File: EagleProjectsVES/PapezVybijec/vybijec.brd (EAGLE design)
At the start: 55.9 x 40.9 mm, 32 parts

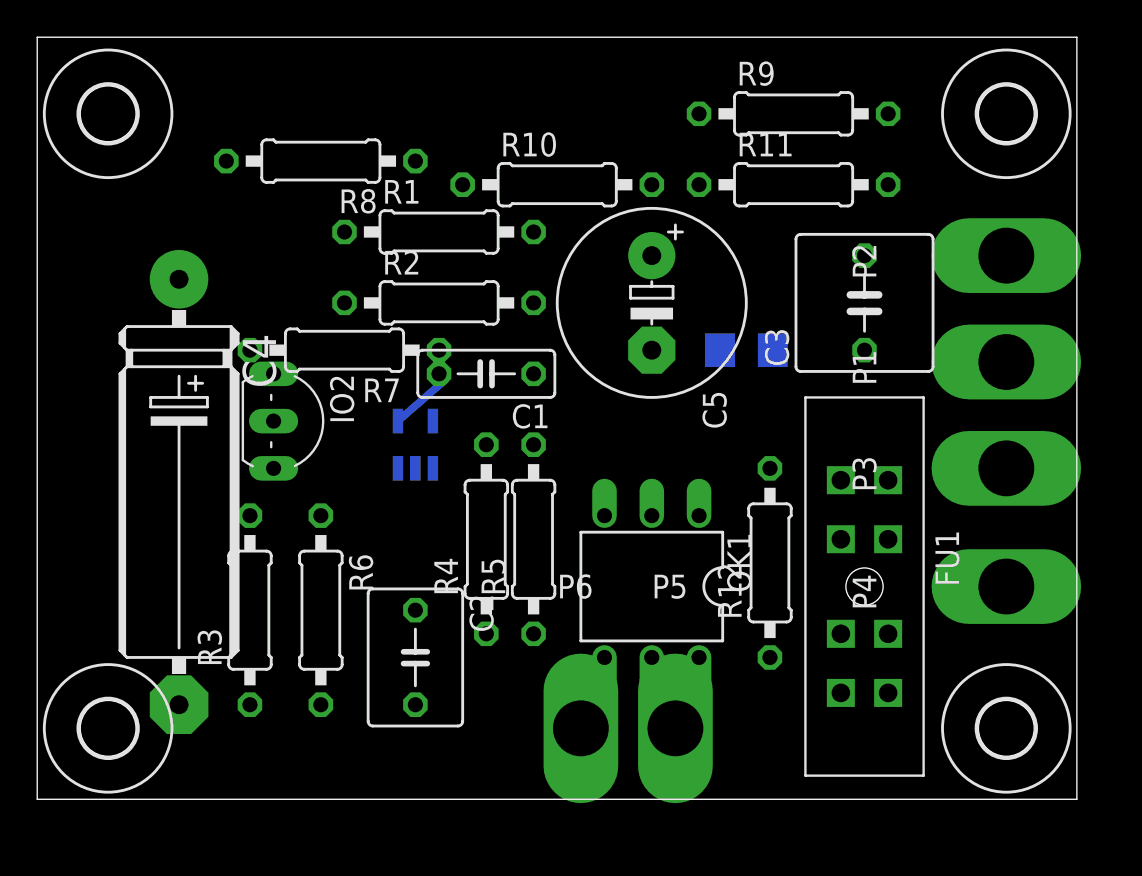
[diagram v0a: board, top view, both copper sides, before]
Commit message: PapezVybijec: - hotova dps
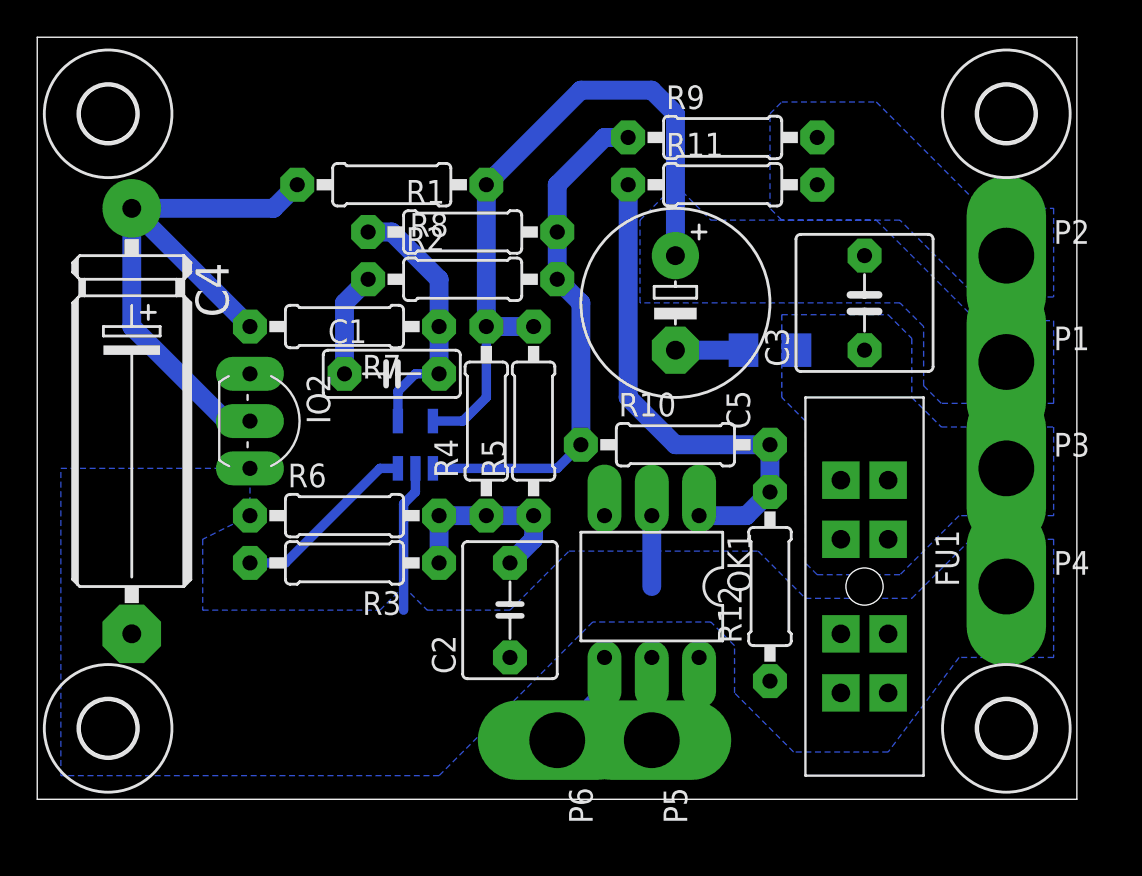
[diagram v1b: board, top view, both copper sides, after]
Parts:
- P1: value (none) -> COLLECTOR
- P2: value (none) -> BASE
- P3: value (none) -> EMITTER
- P4: value (none) -> GROUND
- P5: value (none) -> COL
- P6: value (none) -> EMIT
- moved R10 15.3 mm to (34.3, 19.1)
- moved R4 6.35 mm to (24.1, 20.3)
- moved R5 6.35 mm to (26.7, 20.3)
- moved R3 5.68 mm to (16.5, 12.7), turned to 180 degrees
- moved C2 5.68 mm to (25.4, 10.2), turned to 90 degrees
- moved R6 5.24 mm to (16.5, 15.2), turned to 0 degrees
- moved C1 5.08 mm to (19.1, 22.9), turned to 0 degrees
- moved C4 4.58 mm to (5.08, 20.3)
- moved R9 4.02 mm to (36.8, 35.6)
- moved R8 4.02 mm to (19.1, 33.0)
- moved R11 3.81 mm to (36.8, 33.0)
- moved R2 1.80 mm to (22.9, 27.9)
- moved P6 1.42 mm to (27.9, 3.17), turned to 270 degrees
- moved P5 1.42 mm to (33.0, 3.17), turned to 270 degrees
- moved IO2 1.27 mm to (11.4, 20.3)
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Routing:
- net VCC: track 0.00 -> 37.8 mm
- net N$3: track 0.00 -> 33.2 mm
- net N$2: track 0.00 -> 27.8 mm
- net N$8: track 0.00 -> 27.0 mm
- net GND: track 0.00 -> 11.7 mm
- net N$6: track 0.00 -> 10.7 mm
- net N$4: track 3.83 -> 14.1 mm
- net N$5: track 0.00 -> 10.1 mm
- net N$1: track 0.00 -> 5.61 mm
- net N$11: track 0.00 -> 5.50 mm
- net N$10: track 0.00 -> 4.45 mm
- net N$14: track 0.00 -> 3.66 mm
- added copper zone on layer 16, net GND
- added copper zone on layer 16, net N$7
- added copper zone on layer 16, net N$9
- added copper zone on layer 16, net VCC
